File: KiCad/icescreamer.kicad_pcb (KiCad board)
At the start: 2 copper layers, 60 x 20 mm, 84 parts, among them J1 Audio-Jack-3_3Switches, J2 Audio-Jack-3_3Switches, Q1 2SC1815, Q2 2SC1815, Q20 2SC1815, Q21 2SC1815, Q22 2SC1815, Q23 Q_NJFET_SGD, Q24 Q_NJFET_SGD, SW1 SW_TPDT, SW20 SW_Push, U1 NE5532

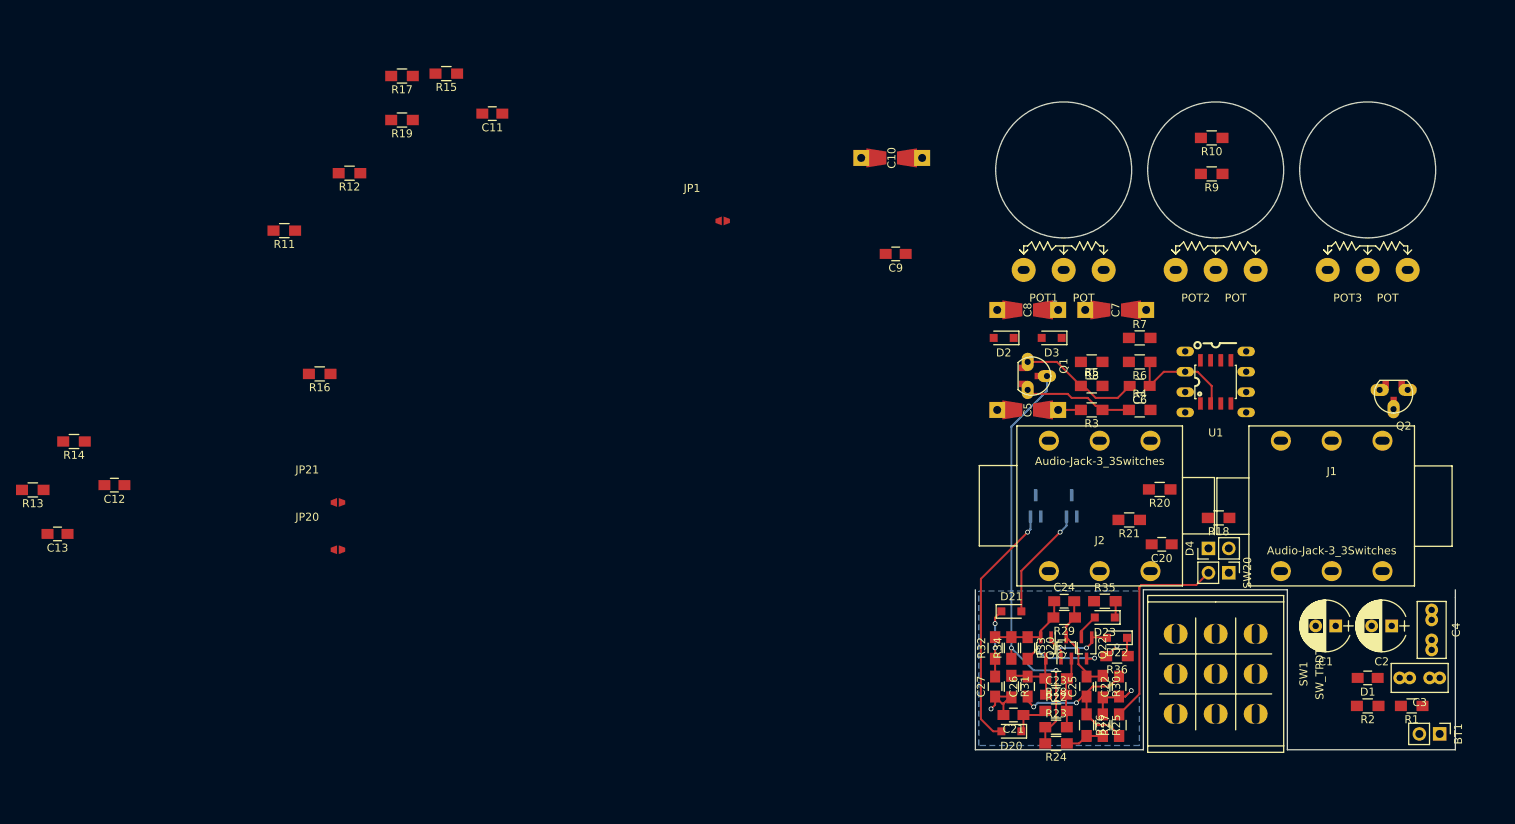
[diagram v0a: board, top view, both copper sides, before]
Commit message: JorFru approved
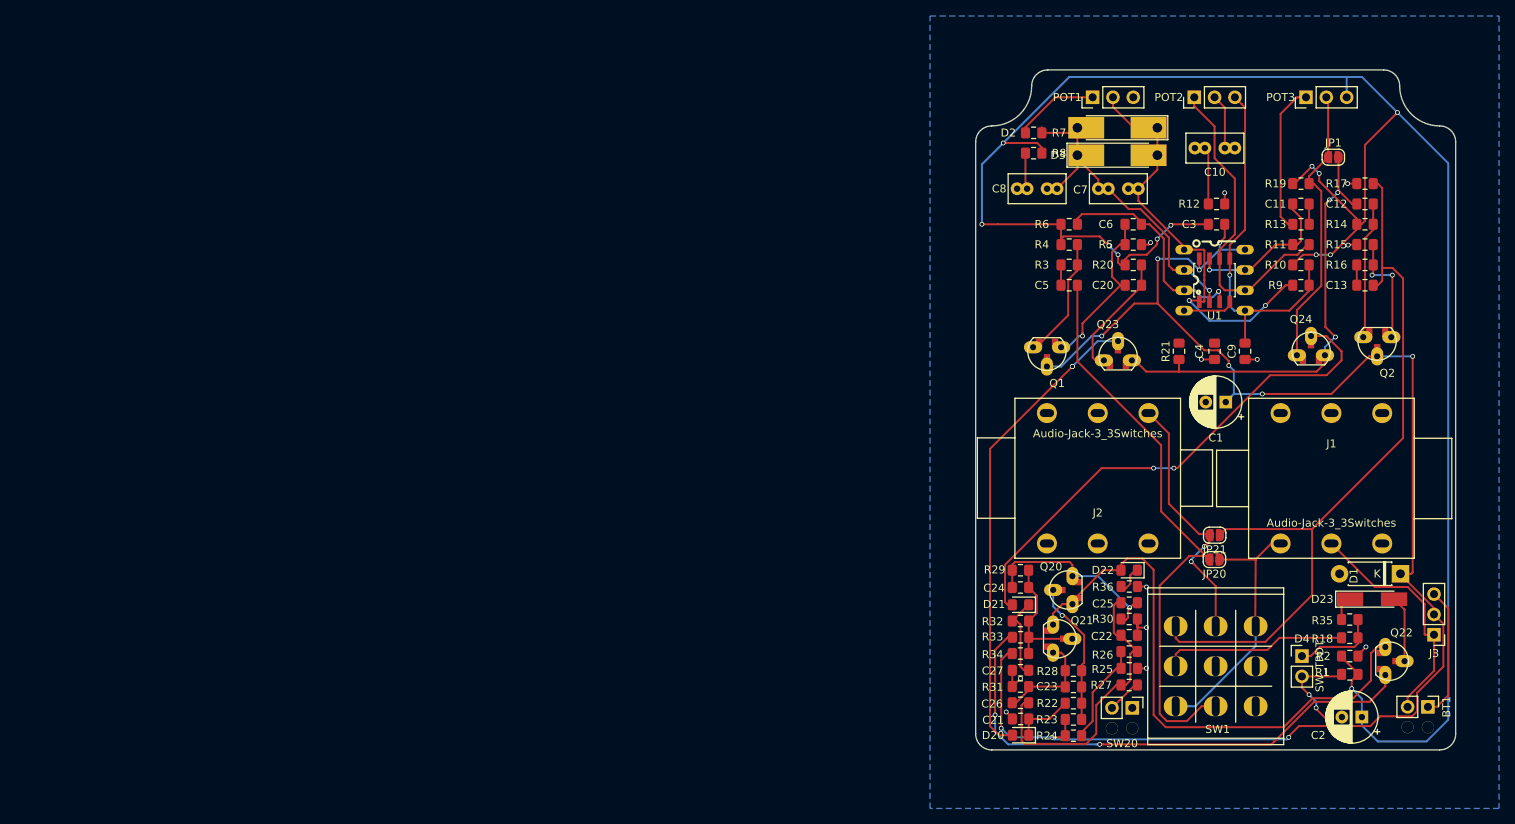
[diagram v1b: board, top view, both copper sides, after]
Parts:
- added J3: Barrel_Jack_Switch, Connector_PinHeader_2.54mm:PinHeader_1x03_P2.54mm_Vertical, F.Cu at (240.8, 125.6)
- BT1, SW20: footprint Socket_Strips:Socket_Strip_Straight_1x02_Pitch2.54mm -> drawdio:1x02_P2.54mm_Hole
- C1, C2: footprint Capacitors_THT:CP_Radial_D6.3mm_P2.50mm -> Capacitor_THT:CP_Radial_D6.3mm_P2.50mm
- C10, C7, C8: footprint drawdio:Resistor_SMD+THT -> Capacitor_THT:C_Rect_L7.0mm_W3.5mm_P2.50mm_P5.00mm
- C11, C12, C13, C20, C21, C22, C23, C24, C25, C26, C27, C6, C9: footprint Capacitors_SMD:C_0805_HandSoldering -> Capacitor_SMD:C_0805_2012Metric_Pad1.15x1.40mm_HandSolder
- C3, C4: footprint Capacitors_THT:C_Rect_L7.0mm_W3.5mm_P2.50mm_P5.00mm -> Capacitor_SMD:C_0805_2012Metric_Pad1.15x1.40mm_HandSolder
- C5: footprint drawdio:Resistor_SMD+THT -> Capacitor_SMD:C_0805_2012Metric_Pad1.15x1.40mm_HandSolder
- D1: footprint Capacitors_SMD:C_0805_HandSoldering -> Diode_THT:D_DO-41_SOD81_P7.62mm_Horizontal
- D2, D3: footprint Diodes_SMD:D_SOD-323_HandSoldering -> Diode_SMD:D_MELF-RM10_Universal_Handsoldering
- D20, D21, D22: footprint Diodes_SMD:D_SOD-323_HandSoldering -> Diode_SMD:D_0805_2012Metric_Pad1.15x1.40mm_HandSolder
- D23: footprint Diodes_SMD:D_SOD-323_HandSoldering -> Diode_SMD:D_MiniMELF_Handsoldering
- D4: footprint Pin_Headers:Pin_Header_Straight_1x02_Pitch2.54mm -> Connector_PinHeader_2.54mm:PinHeader_1x02_P2.54mm_Vertical
- JP1, JP20, JP21: footprint def-footprints:Miscellaneous_Solder_Jumper -> Jumper:SolderJumper-2_P1.3mm_Open_RoundedPad1.0x1.5mm
- POT1, POT2, POT3: footprint footprints:IcePOT -> Connector_PinHeader_2.54mm:PinHeader_1x03_P2.54mm_Vertical
- Q20, Q21, Q22: footprint TO_SOT_Packages_SMD:SOT-323_SC-70_Handsoldering -> drawdio:TO-92_SOT23_JorFru_compact
- Q23, Q24: footprint TO_SOT_Packages_SMD:SOT-323_SC-70_Handsoldering -> drawdio:TO-92_SOT23_JorFru_compact; moved to F.Cu
- R1, R10, R11, R12, R13, R14, R15, R16, R17, R18, R19, R2, R20, R21, R22, R23, R24, R25, R26, R27, R28, R29, R3, R30, R31, R32, R33, R34, R35, R36, R4, R5, R6, R7, R8, R9: footprint Resistors_SMD:R_0805_HandSoldering -> Resistor_SMD:R_0805_2012Metric_Pad1.15x1.40mm_HandSolder
- moved C13 166.4 mm to (232.2, 81.9)
- moved R14 163.6 mm to (232.2, 74.3)
- moved R13 162.0 mm to (224.2, 74.3)
- moved C12 160.2 mm to (232.2, 71.8)
- moved R16 131.4 mm to (232.2, 79.4), turned to 0 degrees
- moved R11 127.1 mm to (224.2, 76.8)
- moved R17 121.1 mm to (232.2, 69.2)
- moved R15 116.8 mm to (232.2, 76.8)
- moved R19 112.6 mm to (224.2, 69.2)
- moved JP21 109.7 mm to (213.4, 113.2)
- moved JP20 109.6 mm to (213.3, 116.2)
- moved R12 108.4 mm to (213.6, 71.8), turned to 0 degrees
- moved C11 101.7 mm to (224.2, 71.8)
- moved JP1 76.7 mm to (228.2, 65.9), turned to 0 degrees
- moved C3 63.2 mm to (213.6, 74.3)
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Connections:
- BT1 pad 1: LED_ANODE -> Net-(BT1-Pad1)
- C1 pad 1: LED_ANODE -> +VDC
- C3 pad 1: LED_ANODE -> +VDC
- D1 pad 1: LED_ANODE -> +VDC
- D4 pad 2: LED_ANODE -> +VDC
- J1 pad 5: Net-(J1-Pad5) -> (no net)
- J1 pad 6: Net-(J1-Pad6) -> (no net)
- J2 pad 4: Net-(J2-Pad4) -> (no net)
- J2 pad 5: Net-(J2-Pad5) -> (no net)
- J2 pad 6: Net-(J2-Pad6) -> (no net)
- POT1 pad 3: Net-(POT1-Pad3) -> (no net)
- Q1 pad 2: LED_ANODE -> +VDC
- Q2 pad 2: LED_ANODE -> +VDC
- R1 pad 1: LED_ANODE -> +VDC
- R23 pad 1: LED_ANODE -> +VDC
- R24 pad 2: LED_ANODE -> +VDC
- R34 pad 1: LED_ANODE -> +VDC
- SW1 pad 32: Net-(SW1-Pad32) -> (no net)
- U1 pad 2: Net-(C6-Pad1) -> Net-(C7-Pad2)
- U1 pad 3: Net-(C7-Pad2) -> Net-(C6-Pad1)
- U1 pad 8: LED_ANODE -> +VDC
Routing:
- net GNDREF: track 0.10 -> 252.1 mm, vias 0 -> 12
- net +VDC: track 0.00 -> 212.5 mm, vias 0 -> 12
- net EFF_OUT: track 0.00 -> 94.8 mm
- net EFF_IN: track 0.00 -> 73.2 mm
- net Net-(D22-Pad2): track 11.7 -> 73.9 mm, vias 2 -> 0
- net PSEUDO_OUT: track 0.00 -> 57.3 mm, vias 0 -> 3
- net Net-(Q22-Pad3): track 10.3 -> 66.8 mm
- net LED_ANODE: track 55.1 -> 0.00 mm, vias 2 -> 0
- net Net-(C7-Pad1): track 0.00 -> 53.2 mm, vias 0 -> 2
- net Net-(D21-Pad2): track 14.2 -> 64.1 mm, vias 1 -> 2
- net Net-(C9-Pad2): track 0.00 -> 45.9 mm, vias 0 -> 1
- net Net-(C7-Pad2): track 0.00 -> 42.2 mm, vias 0 -> 1
- net Net-(POT2-Pad1): track 0.00 -> 40.2 mm
- net PSEUDO_IN_2: track 0.00 -> 35.5 mm
- net JACK_IN: track 0.00 -> 35.0 mm
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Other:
- board size 60 x 20 mm -> 60 x 85 mm
